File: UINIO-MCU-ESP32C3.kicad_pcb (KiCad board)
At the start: 2 copper layers, 59.8 x 20.4 mm, 50 parts, among them J1 Conn_01x15_Male, J2 外接串行下载接口, J3 Conn_01x15_Male, SW1 复位按键, SW2 下载按键, U1 ME6211C33M5G-N, U2 W25Q128JVSSIQ, U3 ESP32-C3, U4 CH343P, Y1 40MHz

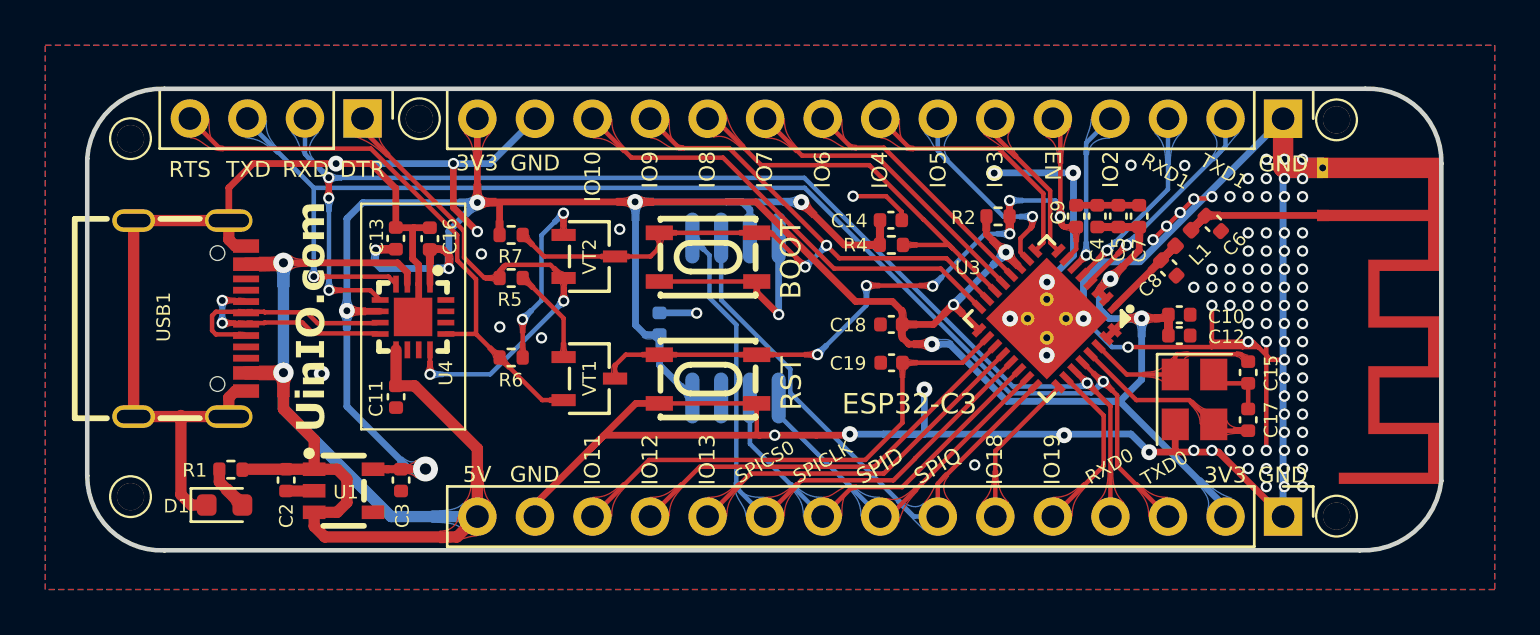
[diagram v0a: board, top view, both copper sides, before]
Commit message: Fix bug.
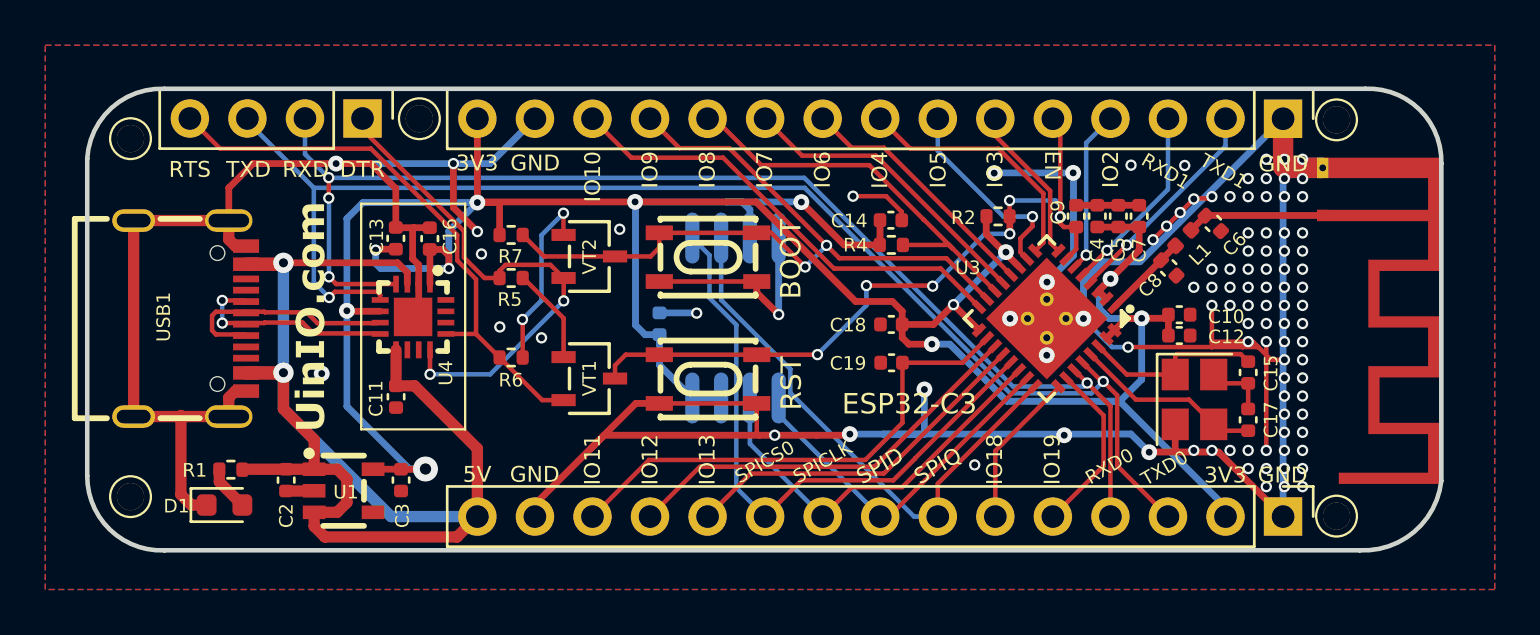
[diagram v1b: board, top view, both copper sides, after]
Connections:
- U4 pad 4: /U0TXD -> /U0RXD
- U4 pad 5: /U0RXD -> /U0TXD
